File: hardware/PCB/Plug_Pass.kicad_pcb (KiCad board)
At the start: 2 copper layers, 152.4 x 114.3 mm, 9 parts, among them J1 Conn_01x06, J10 TDPT-1017503, J2 Conn_01x08, J3 Conn_01x06, J7 Conn_01x06

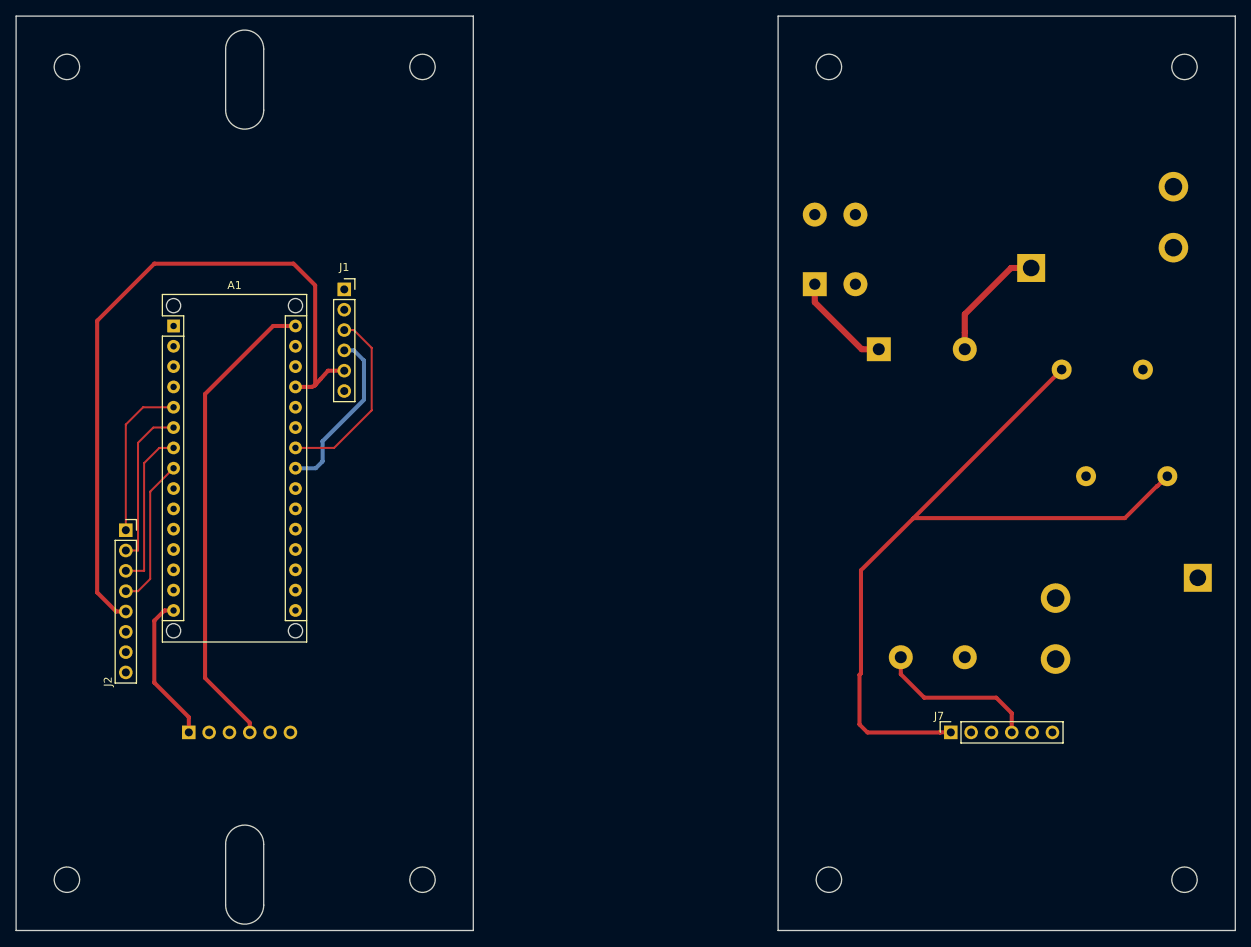
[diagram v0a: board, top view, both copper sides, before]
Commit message: Add files via upload
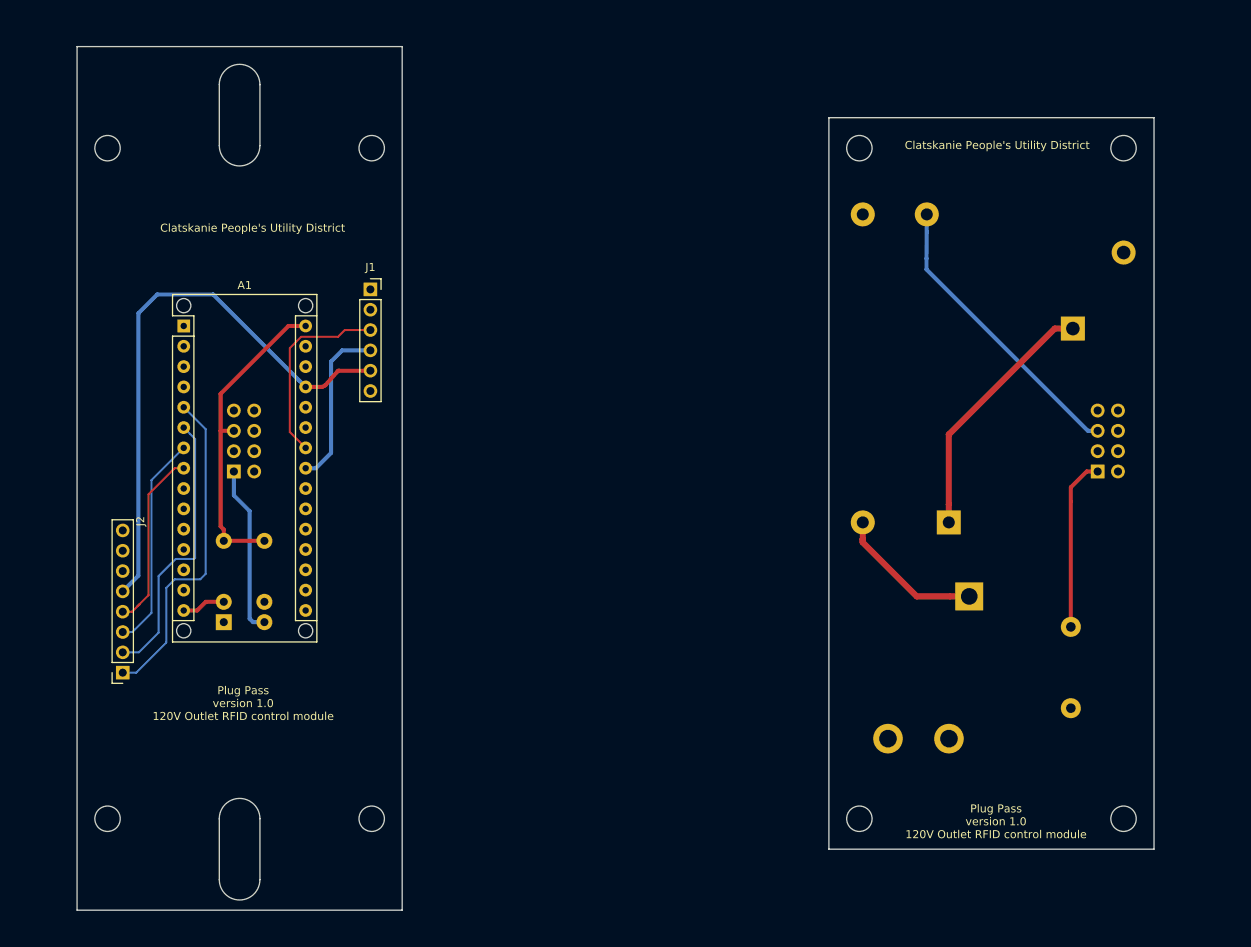
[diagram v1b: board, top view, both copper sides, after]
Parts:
- removed J7: Conn_01x06, Plug_Pass:PinSocket_1x06_P2.54mm_Vertical
- added J4: Conn_02x04_Odd_Even, Plug_Pass:IDC-Header_2x04_P2.54mm_Vertical, B.Cu at (211.4, 95.0)
- J10: footprint Plug_Pass:TDPT_2P_5.08MM -> Plug_Pass:TDPT_2P_6.35MM
- J3: value Conn_01x06 -> Conn_02x04_Odd_Even; footprint Plug_Pass:PinHeader_1x06_P2.54mm_Vertical -> Plug_Pass:IDC-Header_2x04_P2.54mm_Vertical
- RLY2: value T95S5D22-5 -> G5V-1-DC5; footprint Plug_Pass:RLY-T9AS5D22-5 -> Plug_Pass:Relay_THT_G5V-1
- moved RLY2 98.0 mm to (102.2, 113.9), turned to 90 degrees
- moved RLY1 68.6 mm to (181.8, 107.3), turned to 270 degrees
- moved J3 33.1 mm to (103.4, 95.0), turned to 0 degrees
- moved J10 32.7 mm to (208.3, 77.2)
- moved PS1 23.3 mm to (192.8, 101.4), turned to 90 degrees
- moved J2 17.8 mm to (89.5, 120.2), turned to 180 degrees
- moved J1 3.27 mm to (120.5, 72.3)
- moved A1 1.27 mm to (97.2, 76.8)
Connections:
- A1 pad 15: /RelayPin -> Net-(A1-Pad15)
- A1 pad 30: +5V -> VCC
- J10 pad 2: Net-(J10-Pad2) -> GNDREF
- J3 pad 4: +5V -> Net-(J3-Pad4)
- J3 pad 5: Net-(J3-Pad5) -> VCC
- J3 pad 6: GNDREF -> Net-(J3-Pad6)
- PS1 pad 4: +5V -> VCC
- RLY2 pad 2: GNDREF -> Net-(A1-Pad15)
- RLY2 pad 5: /RelayPin -> VCC
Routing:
- net +5V: track 169.2 -> 71.2 mm
- net /RelayPin: track 119.2 -> 42.9 mm
- net VCC: track 0.00 -> 76.1 mm
- net /SCK: track 20.1 -> 41.5 mm
- net Net-(J10-Pad1): track 12.7 -> 32.0 mm
- net /MISO: track 20.2 -> 35.0 mm
- net /MOSI: track 20.2 -> 26.9 mm
- net Net-(A1-Pad15): track 0.00 -> 5.45 mm
- net /SS: track 18.7 -> 22.7 mm
- net Net-(J9-Pad~): track 15.1 -> 18.6 mm
- net /SCL: track 23.6 -> 24.3 mm
- net /SDA: track 21.5 -> 20.9 mm
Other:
- board size 152.4 x 114.3 mm -> 134.6 x 108 mm
- board text added: "Clatskanie People's Utility District"
- board text added: "Plug Pass version 1.0 120V Outlet RFID control module"
